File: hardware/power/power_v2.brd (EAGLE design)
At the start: 92 x 92 mm, 61 parts, among them J1 FASTON1289_ST, J2 FASTON1289_ST, J3 12v, J4 5v, J5 XT30PW-F, J6 XT30PW-F, J7 XT30PW-F, J8 XT30PW-F, Q1 MMBT5401L, Q2 PSMN1R0-40YSH, Q3 MMBT5401L, Q4 PSMN1R0-40YSH, U1 PDQ30-Q24-S5-D, U2 PDQ30-Q24-S12-D

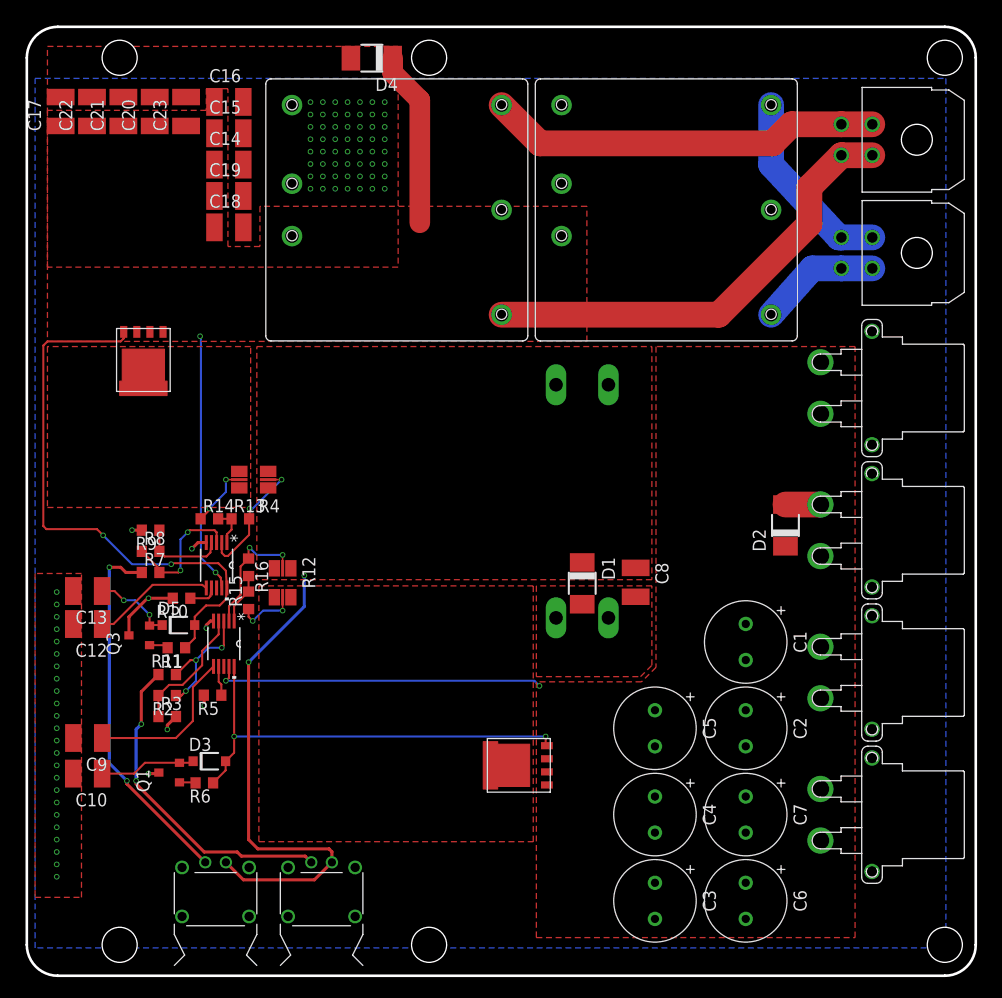
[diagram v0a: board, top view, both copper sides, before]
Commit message: Updates to power board
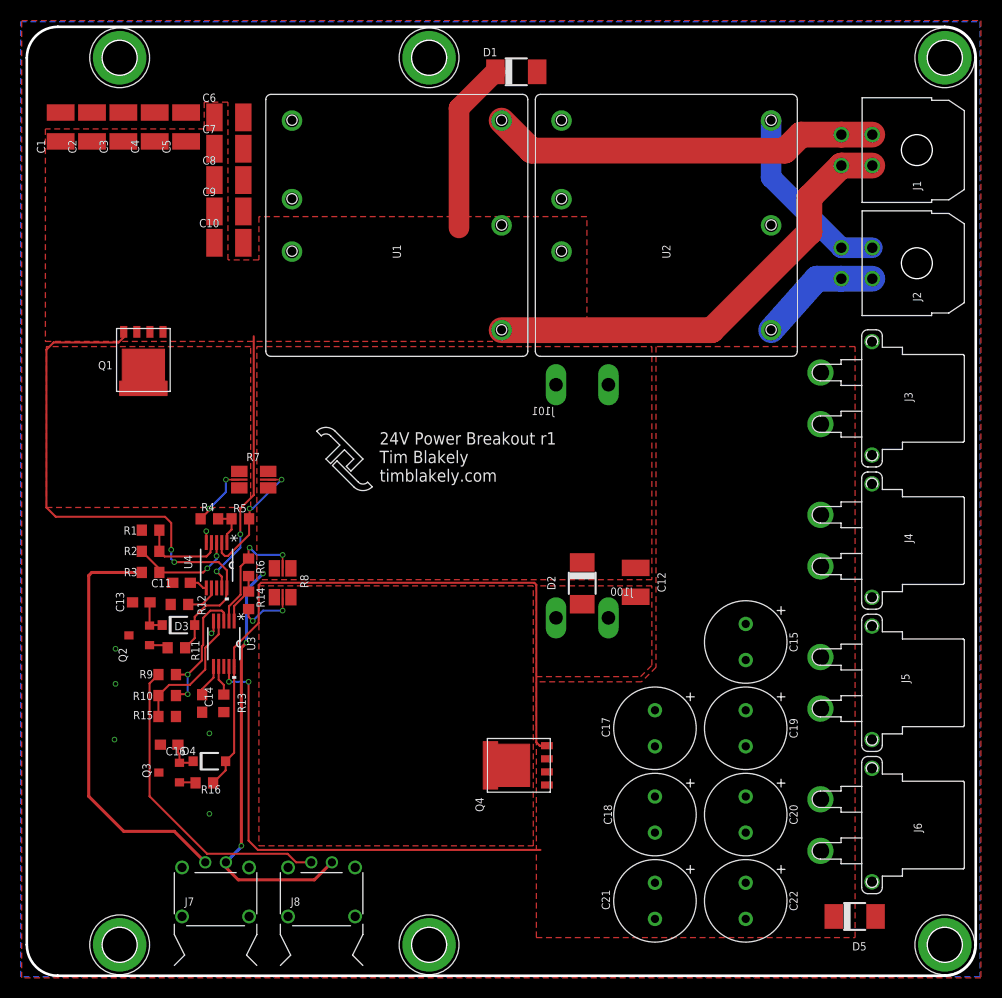
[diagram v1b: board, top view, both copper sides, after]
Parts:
- removed C23: 10uF, timlib:C1210
- removed U$13, U$26: 2-PIN, timlib:M80-8420242
- added C11: 2.2nF, rcl:C0603
- added H1, H2, H3, H4, H5, H6: GND_HOLE_M3, timlib:HOLE_GND_M3
- added J100, J101: FASTON1289_ST, timlib:FASTON_1289-ST
- C1, C2, C3, C4, C5, C6, C7: value 220uf -> 10uF; device timlib:C_ELEC_8X11_5 -> timlib:C1210
- C10: value 16nF -> 10uF
- C12: value 2.2n -> 0.01uF
- C13: value 16nF -> 47nF; device timlib:C1210 -> rcl:C0603
- C14: value 10uF -> 2.2nF; device timlib:C1210 -> rcl:C0603
- C15, C17, C18, C19, C20, C21, C22: value 10uF -> 220uf; device timlib:C1210 -> timlib:C_ELEC_8X11_5
- C16: value 10uF -> 47nF; device timlib:C1210 -> rcl:C0603
- C8: value 0.01uF -> 2.2nF
- C9: value 2.2n -> 10uF
- D1: value SMAJ30A -> SK510A-LTP
- D2: value SK510A-LTP -> SMAJ30A
- D4: value SK510A-LTP -> 1N4148W-7-F; device timlib:DO-214AC -> timlib:SOD123
- D5: value 1N4148W-7-F -> SK510A-LTP; device timlib:SOD123 -> timlib:DO-214AC
- J1: value FASTON1289_ST -> 12v; device timlib:FASTON_1289-ST -> timlib:MOLEX_4_RA
- J2: value FASTON1289_ST -> 5v; device timlib:FASTON_1289-ST -> timlib:MOLEX_4_RA
- J3: value 12v -> XT30PW-F; device timlib:MOLEX_4_RA -> timlib:XT30PW-F
- J4: value 5v -> XT30PW-F; device timlib:MOLEX_4_RA -> timlib:XT30PW-F
- J7, J8: value XT30PW-F -> 2-PIN; device timlib:XT30PW-F -> timlib:M80-8420242
- Q1: value MMBT5401L -> PSMN1R0-40YSH; device timlib:SOT23-3 -> timlib:LFPAK56E
- Q2: value PSMN1R0-40YSH -> MMBT5401L; device timlib:LFPAK56E -> timlib:SOT23-3
- R1: value 47.5k -> 4.32k
- R10: value 18.9k -> 3.4k
- R11: value 18.9 -> 1k
- R12: value PMR25HZPFV1L00 -> 18.9k; device timlib:R1210_KELVIN -> rcl:R0603
- R13: value 10 -> 18.9k
- R15: value 4.53 -> 4.32k
- R16: value 10 -> 1k
- R3, R9: value 4.32k -> 47.5k
- R4: value PMR25HZPFV1L00 -> 4.53; device timlib:R1210_KELVIN -> rcl:R0603
- R5: value 18.9k -> 10
- R6: value 18.9 -> 10
- R7: value 47.5k -> 0.002; device rcl:R0603 -> timlib:R1210_KELVIN
- R8: value 3.4k -> 0.002; device rcl:R0603 -> timlib:R1210_KELVIN
- U1: value PDQ30-Q24-S5-D -> PDQ30-Q24-S12-D
- U2: value PDQ30-Q24-S12-D -> PDQ30-Q24-S5-D
- moved C22 99.4 mm to (69.7, 7.26), turned to 270 degrees
- moved C21 92.3 mm to (60.9, 7.26), turned to 270 degrees
- moved C3 91.0 mm to (9.36, 82.3), turned to 90 degrees
- moved C6 91.0 mm to (19.6, 83.2), turned to 0 degrees
- moved C20 89.0 mm to (69.7, 15.6), turned to 270 degrees
- moved C2 86.1 mm to (6.32, 82.3), turned to 90 degrees
- moved C1 83.1 mm to (3.28, 82.3), turned to 90 degrees
- moved C17 83.0 mm to (60.9, 24.0), turned to 270 degrees
- moved C4 82.4 mm to (12.4, 82.3), turned to 90 degrees
- moved C7 81.7 mm to (19.6, 80.2), turned to 0 degrees
- moved C5 73.9 mm to (15.4, 82.3), turned to 90 degrees
- moved C19 71.9 mm to (69.7, 24.0), turned to 270 degrees
- moved D5 71.4 mm to (80.3, 5.75)
- moved C18 70.3 mm to (60.9, 15.6), turned to 270 degrees
- moved C15 70.3 mm to (69.7, 32.4), turned to 270 degrees
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- renumbered U$1 to U3, U$14 to U4
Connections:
- net +12VOUT: now also J1.CIRCUIT2, J1.CIRCUIT4, U1.P$3; no longer J3.CIRCUIT2, J3.CIRCUIT4, U2.P$3
- net +24V_BATT: now also C12.1, D2.C, J101.P$1, J101.P$2, J7.1, J8.1, R7.1A, R7.1B, R8.1A, R8.1B; no longer C8.1, D1.C, J1.P$1, J1.P$2, R12.1A, R12.1B, R4.1A, R4.1B, U$13.1, U$26.1
- net +24V_ISO: now also C1.1, C10.1, C2.1, C3.1, C4.1, C5.1, C6.1, C7.1, C8.1, C9.1, D1.C, Q1.1, Q1.2, Q1.3; no longer C14.1, C15.1, C16.1, C17.1, C18.1, C19.1, C20.1, C21.1, C22.1, C23.1, D4.C, Q4.1, Q4.2, Q4.3
- net +24V_POWER: now also C15.1, C17.1, C18.1, C19.1, C20.1, C21.1, C22.1, D5.C, J3.P$2, J4.P$2, Q4.1, Q4.2, Q4.3; no longer C1.1, C2.1, C3.1, C4.1, C5.1, C6.1, C7.1, D2.C, J7.P$2, J8.P$2, Q2.1, Q2.2, Q2.3
- net +5VOUT: now also J2.CIRCUIT2, J2.CIRCUIT4, U2.P$3; no longer J4.CIRCUIT2, J4.CIRCUIT4, U1.P$3
- net 12V_GND: now also J1.CIRCUIT1, J1.CIRCUIT3, U1.P$5; no longer J3.CIRCUIT1, J3.CIRCUIT3, U2.P$5
- net 5V_GND: now also J2.CIRCUIT1, J2.CIRCUIT3, U2.P$5; no longer J4.CIRCUIT1, J4.CIRCUIT3, U1.P$5
- net GND_BATT: now also C11.2, D5.A, H1.P$1, H2.P$1, H3.P$1, H4.P$1, H5.P$1, H6.P$1, J100.P$1, J100.P$2, J3.P$1, J4.P$1, Q2.C, R1.2, R12.2, R13.2, R15.2; no longer C23.2, D4.A, J2.P$1, J2.P$2, J7.P$1, J8.P$1, Q1.C, R10.2, R3.2, R5.2, R9.2
- net MOSFET_DRAIN: now also Q4.5, R8.2A, R8.2B; no longer Q2.5, R12.2A, R12.2B
- net MOSFET_DRAIN1: now also Q1.5, R7.2A, R7.2B; no longer Q4.5, R4.2A, R4.2B
- net N$1: now also R10.1, R9.2; no longer R1.2, R2.1
- net N$10: now also R14.2, R6.2; no longer R15.2, R16.2
- net N$11: now also R14.1, R8.2_KELVIN; no longer R12.2_KELVIN, R15.1
- net N$12: now also R1.1, R2.2; no longer R8.2, R9.1
- net N$13: now also J7.2, R3.1; no longer R7.1, U$13.2
- net N$14: now also D3.A, Q1.4; no longer D5.A, Q4.4
- net N$15: now also R12.1; no longer R10.1
- net N$16: now also C11.1; no longer C12.1
- net N$17: now also D3.C, Q2.E; no longer D5.C, Q3.E
- net N$18: now also Q2.B; no longer Q3.B
- net N$19: now also R6.1, R8.1_KELVIN; no longer R12.1_KELVIN, R16.1
- net N$2: now also R10.2, R15.1; no longer R2.2, R3.1
- net N$20: now also R4.2, R5.1; no longer R13.1, R14.2
- net N$21: now also R4.1, R7.2_KELVIN; no longer R14.1, R4.2_KELVIN
- net N$22: now also R5.2, R7.1_KELVIN; no longer R13.2, R4.1_KELVIN
- net N$3: now also J8.2, R9.1; no longer R1.1, U$26.2
- net N$4: now also R2.1, R3.2; no longer R7.2, R8.1
- net N$5: now also D4.A, Q4.4, R16.1; no longer D3.A, Q2.4, R6.1
- net N$6: now also R13.1; no longer R5.1
- net N$7: now also C14.1; no longer C9.1
- net N$8: now also C16.1, D4.C, Q3.E; no longer C10.1, D3.C, Q1.E
- net N$9: now also Q3.B, R16.2; no longer Q1.B, R6.2
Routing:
- net N$5: track 43.3 -> 64.5 mm, vias 2 -> 0
- net +24V_POWER: track 32.1 -> 47.5 mm
- net GND_BATT: track 17.6 -> 2.37 mm, vias 87 -> 7
- net N$7: track 15.6 -> 3.20 mm
- net N$16: track 11.8 -> 1.76 mm
- net +24V_BATT: track 49.1 -> 41.5 mm, vias 2 -> 3
- net N$8: track 9.32 -> 3.20 mm
- net N$13: track 35.8 -> 40.6 mm, vias 2 -> 0
- net N$17: track 7.85 -> 3.52 mm, vias 2 -> 0
- net N$4: track 12.8 -> 10.4 mm
- net N$3: track 31.6 -> 30.5 mm, vias 2 -> 0
- net N$1: track 12.7 -> 13.5 mm, vias 3 -> 2
- net 5V_GND: track 18.7 -> 18.2 mm
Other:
- board text added: "24V Power Breakout r1 Tim Blakely timblakely.com"
